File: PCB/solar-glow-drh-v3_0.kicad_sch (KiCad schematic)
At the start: 59 parts, among them J1 UPDI hdr, Q1 BCP5316MTWG, SW2 LED master, U1 AVR64DD28 (VQFN28), U2 ALD910025SALI, U3 LIS2DH12, U4 TLV3011BIDBVR, U5 NT3H2211, U6 TPS22918

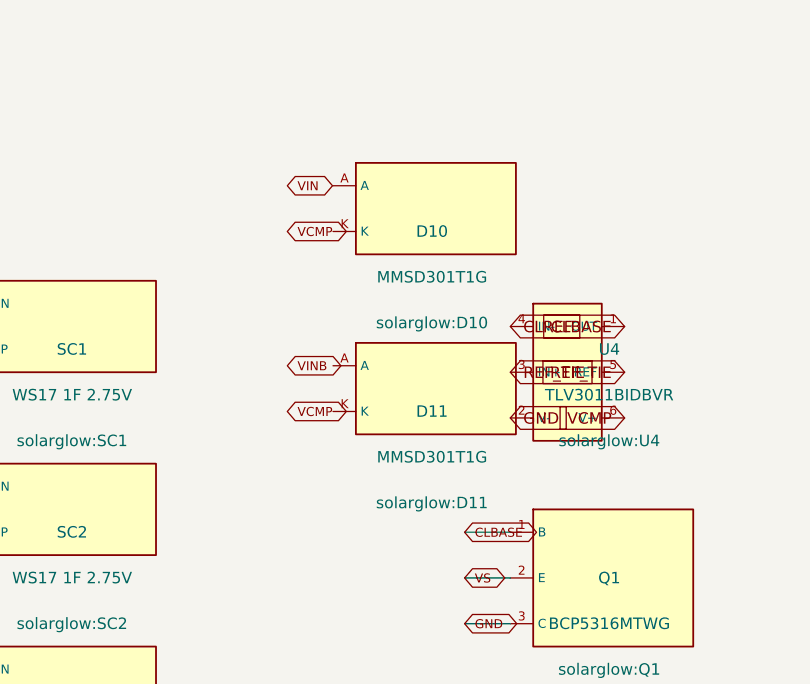
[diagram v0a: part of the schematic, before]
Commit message: Add files via upload
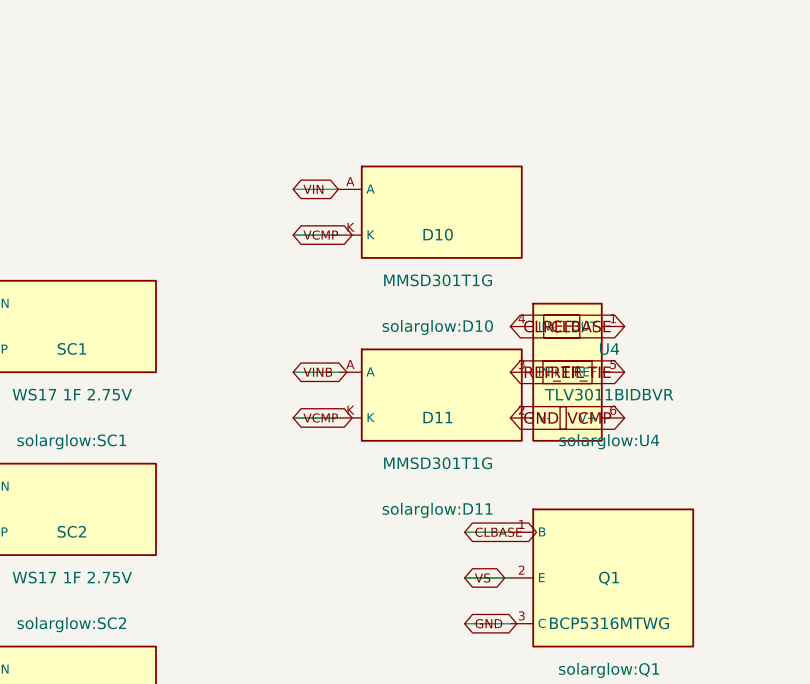
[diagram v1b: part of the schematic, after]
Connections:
- net VCMP: now also D10.K, D11.K
- net VIN: now also D10.A
- net VINB: now also D11.A
